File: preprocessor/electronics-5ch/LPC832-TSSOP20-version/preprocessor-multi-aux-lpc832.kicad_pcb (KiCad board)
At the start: 2 copper layers, 17 x 24 mm, 15 parts, among them P1 ST-IN, P2 ST-OUT, P3 TH-IN, P4 TH-OUT, P5 AUX-IN, P6 LIGHT CONTROLLER, P7 AUX2-IN, P8 AUX3-IN, U1 MCP1703T-3302E/CB, U2 LPC832M101FDH20

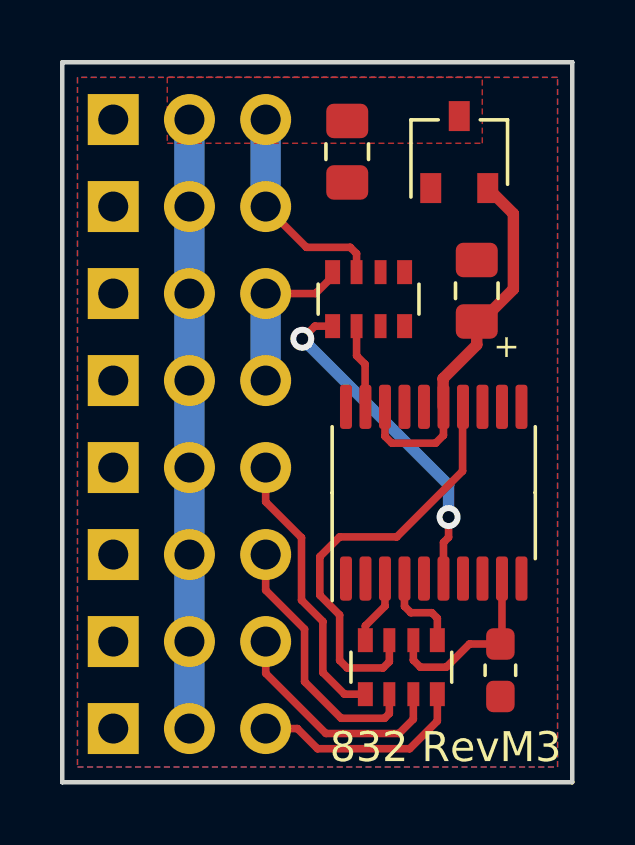
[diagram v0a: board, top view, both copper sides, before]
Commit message: Improve the layout
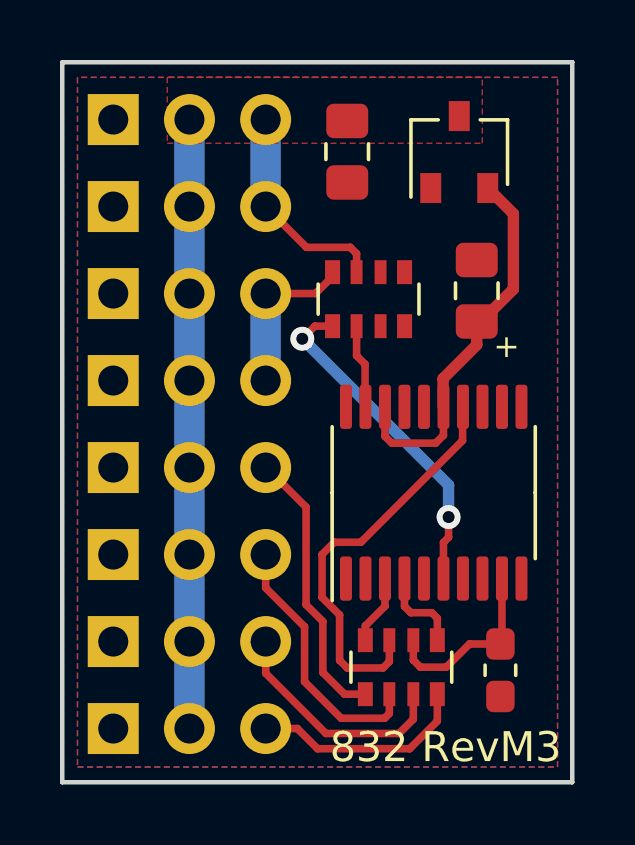
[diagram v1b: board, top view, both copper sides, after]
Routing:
- net /AUX2: track 14.4 -> 13.7 mm

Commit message: Improve FAB layer and silkscreen
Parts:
- RN1, RN2: value R_Pack04 -> 1K

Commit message: Add Gerber for LPC832 variants
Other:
- rule pad_to_mask_clearance: 0.0254 -> 0
